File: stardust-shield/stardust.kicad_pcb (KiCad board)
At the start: 2 copper layers, 154.3 x 139.1 mm, 16 parts, among them J1 BEXUS 28V, J2 Pololu J8557, J3 Pololu J9251, J4 DS3231M, U5 DS18B20, U6 DS18B20, U8 DHT22, U9 SSCDRNN015PASA5

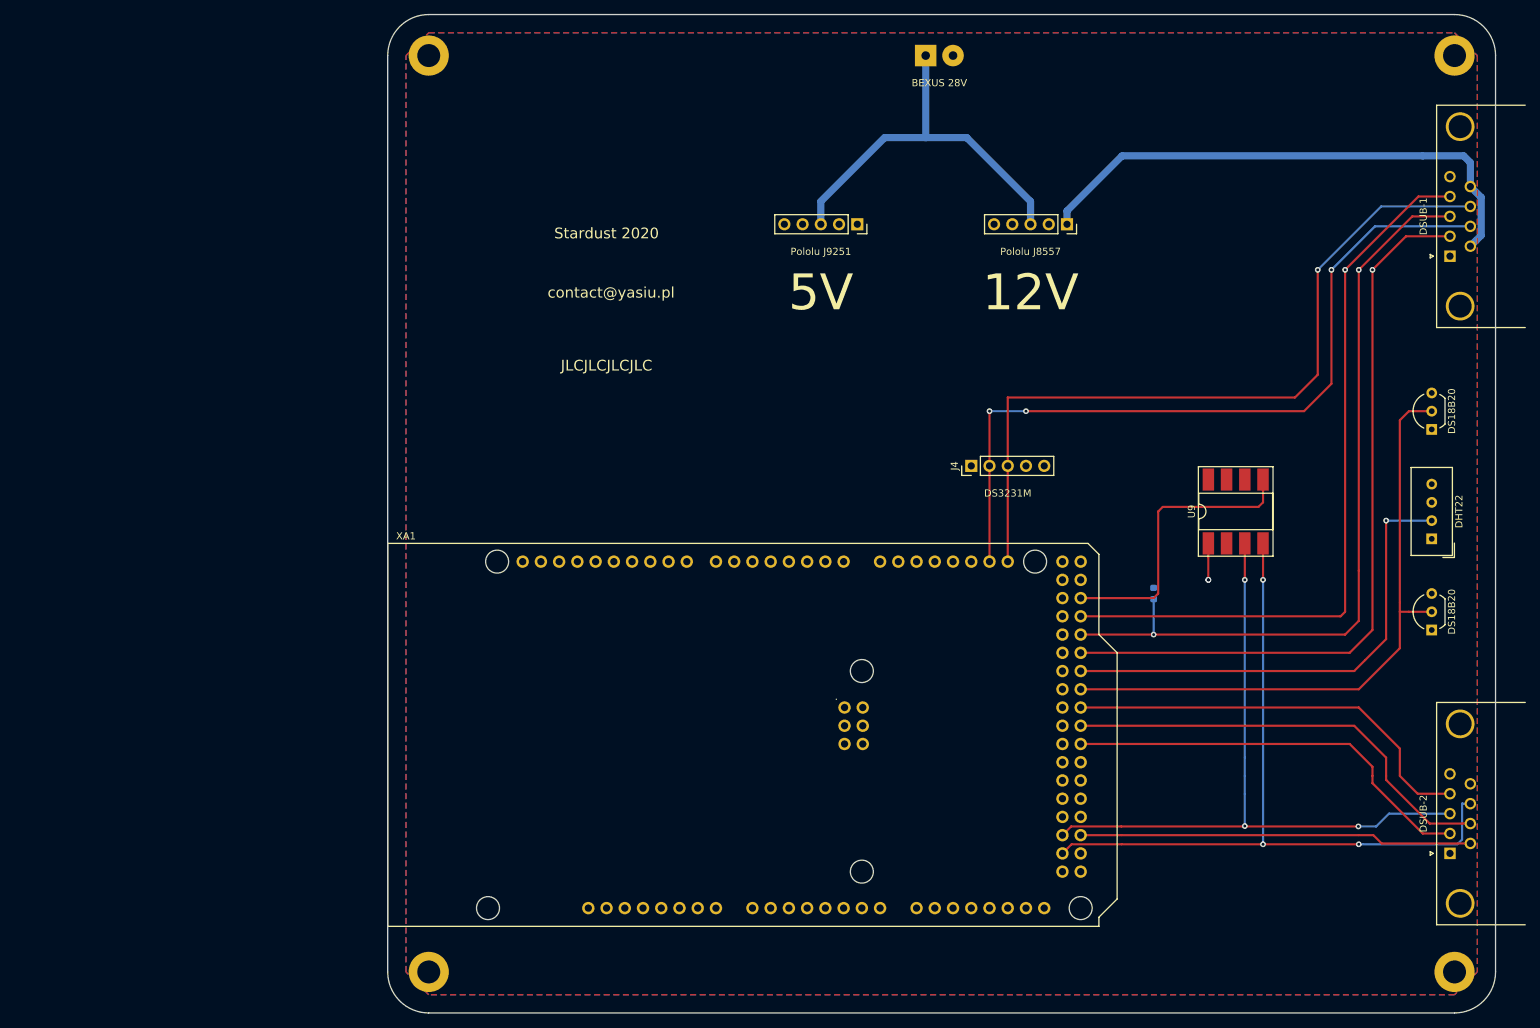
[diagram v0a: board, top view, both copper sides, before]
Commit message: rev.2 init
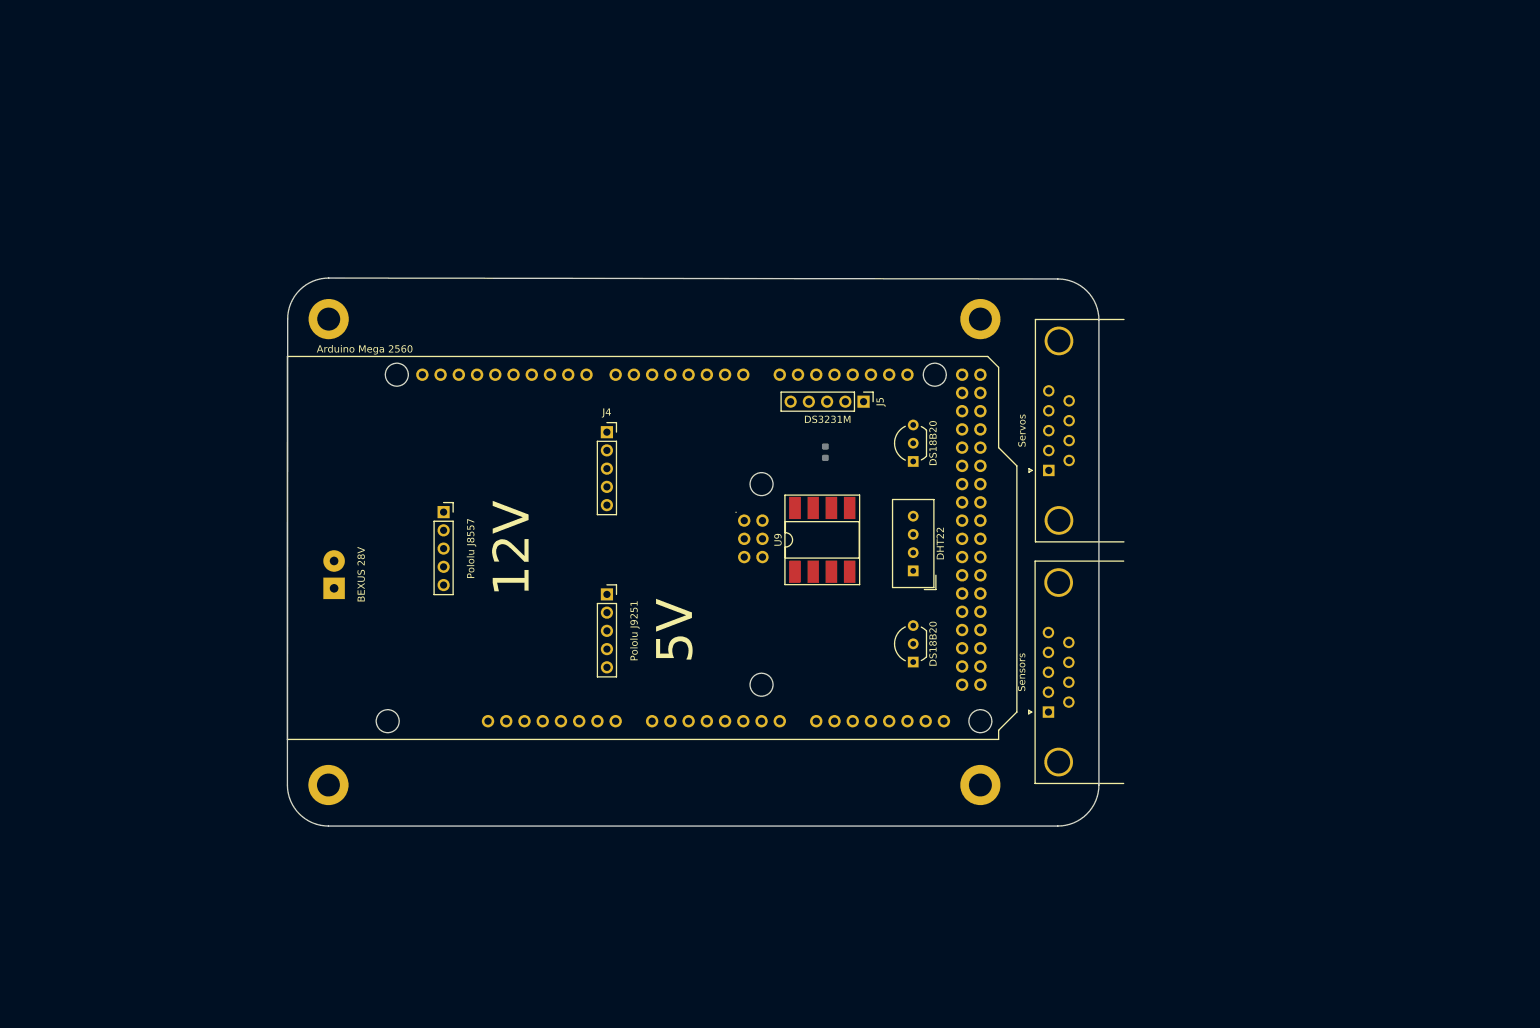
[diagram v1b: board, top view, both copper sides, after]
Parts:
- removed the REF** at (88.9, 151.1)
- removed the REF** at (231.8, 151.1)
- removed the REF** at (88.9, 23.5)
- removed the REF** at (231.8, 23.5)
- added J4: Pololu J9251 Servo, Connector_PinSocket_2.54mm:PinSocket_1x05_P2.54mm_Vertical, F.Cu at (113.7, 76.0)
- added REF**: MountingHole_3.2mm_M3_DIN965_Pad, MountingHole:MountingHole_3.2mm_M3_DIN965_Pad, F.Cu at (165.7, 125.1)
- added REF**: MountingHole_3.2mm_M3_DIN965_Pad, MountingHole:MountingHole_3.2mm_M3_DIN965_Pad, F.Cu at (165.7, 60.2)
- added REF**: MountingHole_3.2mm_M3_DIN965_Pad, MountingHole:MountingHole_3.2mm_M3_DIN965_Pad, F.Cu at (75.0, 60.2)
- added REF**: MountingHole_3.2mm_M3_DIN965_Pad, MountingHole:MountingHole_3.2mm_M3_DIN965_Pad, F.Cu at (74.9, 125.1)
- Arduino Mega 2560: renamed from XA1
- moved J1 110.9 mm to (75.7, 97.7), turned to 90 degrees
- moved J2 95.6 mm to (91.0, 87.1), turned to 0 degrees
- moved U5 72.4 mm to (156.4, 80.0)
- moved U6 72.4 mm to (156.4, 108.0)
- moved U8 72.4 mm to (156.4, 95.3)
- moved Servos 63.4 mm to (175.3, 81.3)
- moved J3 62.2 mm to (113.7, 98.5), turned to 0 degrees
- moved Sensors 59.3 mm to (175.2, 114.9)
- moved U9 57.7 mm to (143.7, 91.0)
- moved R1 49.8 mm to (144.1, 78.7)
- moved Arduino Mega 2560 29.5 mm to (69.2, 118.7)
- moved J5 17.5 mm to (149.5, 71.7), turned to 270 degrees
- renumbered J4 to J5, DSUB-2 to Sensors, DSUB-1 to Servos
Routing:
- net Pump-GPIO: track 109.1 -> 0.00 mm, vias 2 -> 0
- net I2C-SDA: track 107.9 -> 0.00 mm, vias 3 -> 0
- net I2C-SCL: track 106.9 -> 0.00 mm, vias 1 -> 0
- net 1Wire-1: track 104.9 -> 0.00 mm, vias 1 -> 0
- net SPI-CLK: track 104.5 -> 0.00 mm, vias 3 -> 0
- net DHT22-1: track 103.6 -> 0.00 mm, vias 1 -> 0
- net SPI-MISO: track 94.6 -> 0.00 mm, vias 3 -> 0
- net 1Wire-3: track 88.0 -> 0.00 mm
- net +12V: track 74.5 -> 0.00 mm
- net DHT22-3: track 67.2 -> 0.00 mm, vias 1 -> 0
- net SPI-SS-Pressure-1: track 61.7 -> 0.00 mm
- net 1Wire-2: track 58.6 -> 0.00 mm
- net DHT22-2: track 57.9 -> 0.00 mm
- net +28V: track 55.0 -> 0.00 mm
- net SPI-MOSI: track 54.8 -> 0.00 mm
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- removed copper zone on F.Cu, net +5V
- removed copper zone on B.Cu, net GND
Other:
- board size 154.3 x 139.1 mm -> 113 x 76.3 mm

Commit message: 2.0
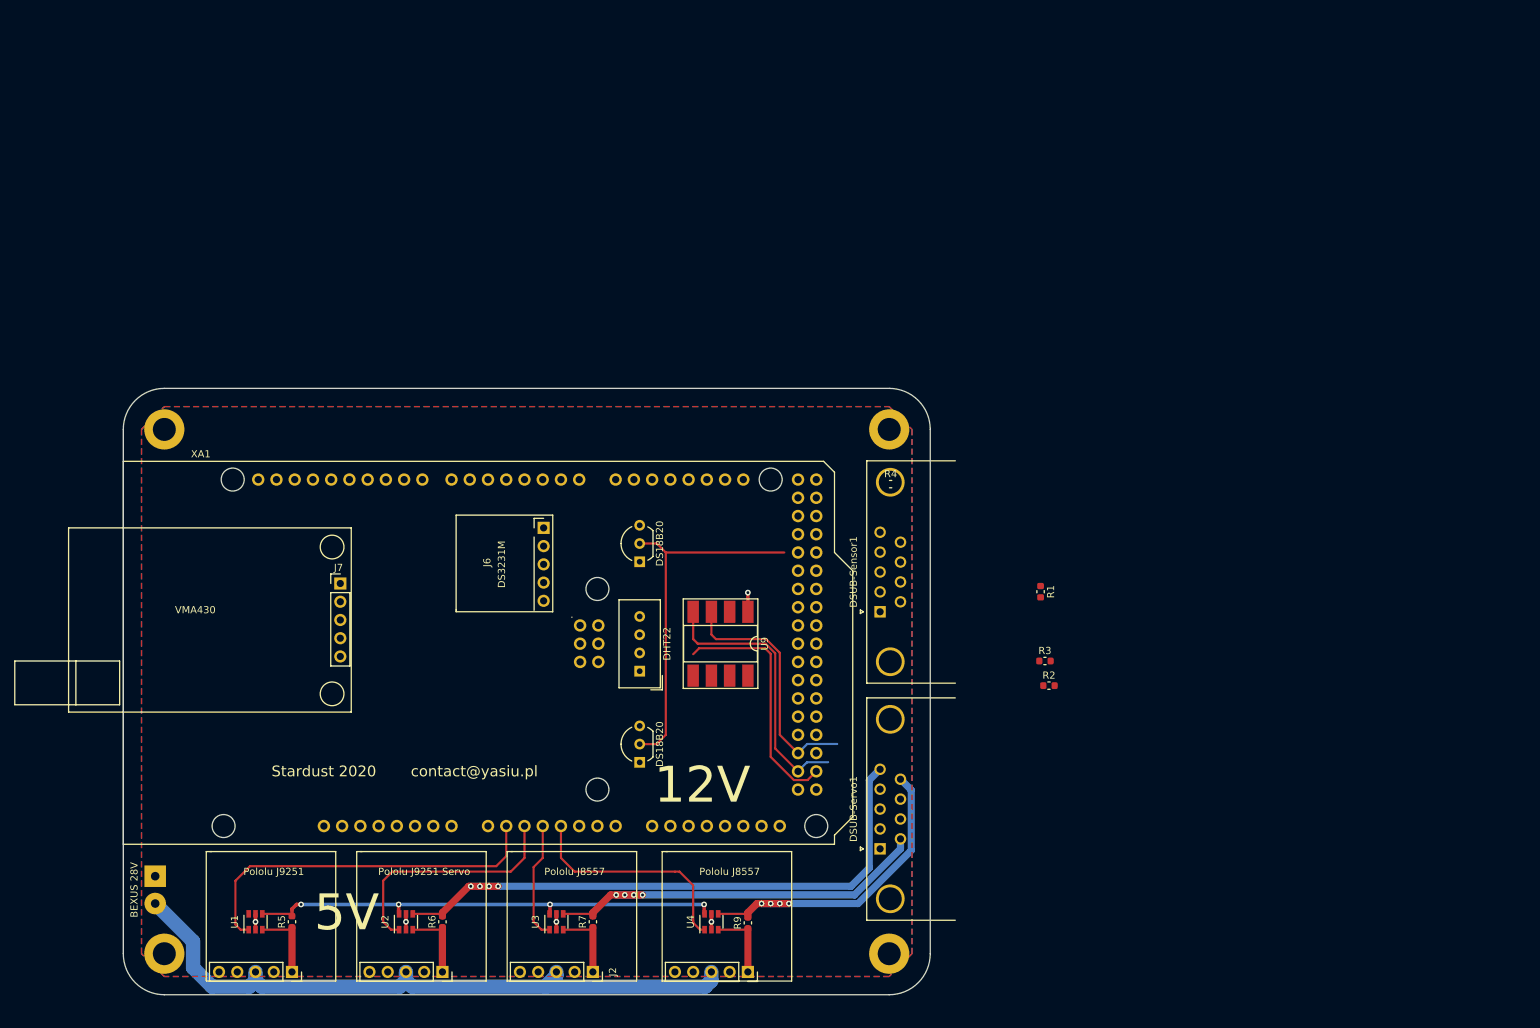
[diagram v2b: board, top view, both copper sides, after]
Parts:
- removed the REF** at (165.7, 125.1)
- removed the REF** at (165.7, 60.2)
- removed the REF** at (75.0, 60.2)
- removed the REF** at (74.9, 125.1)
- added J5: Pololu J9251 Servo, Connector_PinSocket_2.54mm:PinSocket_1x05_P2.54mm_Vertical, F.Cu at (90.8, 151.1)
- added J7: VMA430, Connector_PinHeader_2.54mm:PinHeader_1x05_P2.54mm_Vertical, F.Cu at (76.3, 97.2)
- added R2: 4.7k, Resistor_SMD:R_0603_1608Metric, F.Cu at (175.3, 111.3)
- added R3: 4.7k, Resistor_SMD:R_0603_1608Metric, F.Cu at (174.7, 107.8)
- added R4: 4.7k, Resistor_SMD:R_0603_1608Metric, F.Cu at (153.2, 83.2)
- added R5: 200m, Resistor_SMD:R_0603_1608Metric, F.Cu at (69.8, 144.1)
- added R6: 200m, Resistor_SMD:R_0603_1608Metric, F.Cu at (90.8, 144.1)
- added R7: 200m, Resistor_SMD:R_0603_1608Metric, F.Cu at (111.8, 144.1)
- added R9: 200m, Resistor_SMD:R_0603_1608Metric, F.Cu at (133.3, 144.3)
- added REF**: MountingHole_3.2mm_M3_DIN965_Pad, MountingHole:MountingHole_3.2mm_M3_DIN965_Pad, F.Cu at (153.0, 148.6)
- added REF**: MountingHole_3.2mm_M3_DIN965_Pad, MountingHole:MountingHole_3.2mm_M3_DIN965_Pad, F.Cu at (153.0, 75.6)
- added REF**: MountingHole_3.2mm_M3_DIN965_Pad, MountingHole:MountingHole_3.2mm_M3_DIN965_Pad, F.Cu at (52.1, 148.6)
- added REF**: MountingHole_3.2mm_M3_DIN965_Pad, MountingHole:MountingHole_3.2mm_M3_DIN965_Pad, F.Cu at (52.1, 75.6)
- added U1: INA181, Package_TO_SOT_SMD:SOT-23-6, F.Cu at (64.8, 144.1)
- added U2: INA181, Package_TO_SOT_SMD:SOT-23-6, F.Cu at (85.7, 144.1)
- added U3: INA181, Package_TO_SOT_SMD:SOT-23-6, F.Cu at (106.7, 144.1)
- added U4: INA181, Package_TO_SOT_SMD:SOT-23-6, F.Cu at (128.3, 144.1)
- J3: value Pololu J9251 -> Pololu J8557
- J4: value Pololu J9251 Servo -> Pololu J9251
- J6: renamed from J5; footprint Connector_PinHeader_2.54mm:PinHeader_1x05_P2.54mm_Vertical -> Socket:RTC-DS3231M
- R1: moved to F.Cu
- XA1: renamed from Arduino Mega 2560
- moved J4 87.0 mm to (69.8, 151.1), turned to 270 degrees
- moved J2 67.3 mm to (111.8, 151.1), turned to 270 degrees
- moved DSUB-Servo1 57.7 mm to (151.8, 134.0)
- moved J3 56.1 mm to (133.3, 151.1), turned to 270 degrees
- moved J6 54.7 mm to (99.6, 94.1)
- moved J1 47.2 mm to (50.8, 137.8), turned to 270 degrees
- moved U5 40.6 mm to (118.3, 94.0)
- moved U6 40.6 mm to (118.3, 121.9)
- moved U8 40.6 mm to (118.3, 109.2)
- moved R1 35.7 mm to (174.1, 98.2), turned to 270 degrees
- moved DSUB-Sensor1 27.3 mm to (151.8, 101.0)
- moved XA1 27.1 mm to (46.4, 133.3)
- moved U9 20.2 mm to (129.5, 105.4), turned to 270 degrees
- renumbered Sensors to DSUB-Sensor1, Servos to DSUB-Servo1
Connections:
- net Net-(XA1-PadD16) renamed TX2
- net Net-(XA1-PadD17) renamed RX2
- net Net-(XA1-PadD18) renamed TX1
- net Net-(XA1-PadD19) renamed RX1
- DSUB-Servo1 pad 5: +5V -> +5P
- DSUB-Servo1 pad 9: +12V -> +12P
- J1 pad 1: +28V -> GND
- J1 pad 2: GND -> +28V
- J2 pad 1: +12V -> Net-(J2-Pad1)
- J3 pad 1: +5V -> Net-(J3-Pad1)
- J4 pad 1: +5V -> Net-(J4-Pad1)
- XA1 pad A1: Net-(XA1-PadA1) -> INA1
- XA1 pad A2: Net-(XA1-PadA2) -> INA2
- XA1 pad A3: Net-(XA1-PadA3) -> INA3
- XA1 pad A4: Net-(XA1-PadA4) -> INA4
- XA1 pad D14: Net-(XA1-PadD14) -> TX3
- XA1 pad D15: Net-(XA1-PadD15) -> RX3
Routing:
- net +28V: track 0.00 -> 92.5 mm
- net +5P: track 0.00 -> 85.0 mm, vias 0 -> 4
- net +5V: track 0.00 -> 67.1 mm, vias 0 -> 4
- net +12V: track 0.00 -> 56.3 mm, vias 0 -> 4
- net INA1: track 0.00 -> 51.6 mm
- net 1Wire-3: track 0.00 -> 50.2 mm
- net +12P: track 0.00 -> 45.6 mm, vias 0 -> 4
- net SPI-CLK: track 0.00 -> 38.5 mm
- net SPI-MISO: track 0.00 -> 34.8 mm
- net Net-(XA1-PadD53): track 0.00 -> 34.0 mm
- net INA2: track 0.00 -> 33.8 mm
- net INA4: track 0.00 -> 31.8 mm
- net INA3: track 0.00 -> 16.5 mm
- net GND: track 0.00 -> 11.5 mm, vias 0 -> 5
- net Net-(J5-Pad1): track 0.00 -> 10.5 mm
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- added copper zone on F.Cu, net +5V
- added copper zone on B.Cu, net GND
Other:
- board size 113 x 76.3 mm -> 112.4 x 84.5 mm
